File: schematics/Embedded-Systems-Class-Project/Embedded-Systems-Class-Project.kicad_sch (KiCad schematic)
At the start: 16 parts

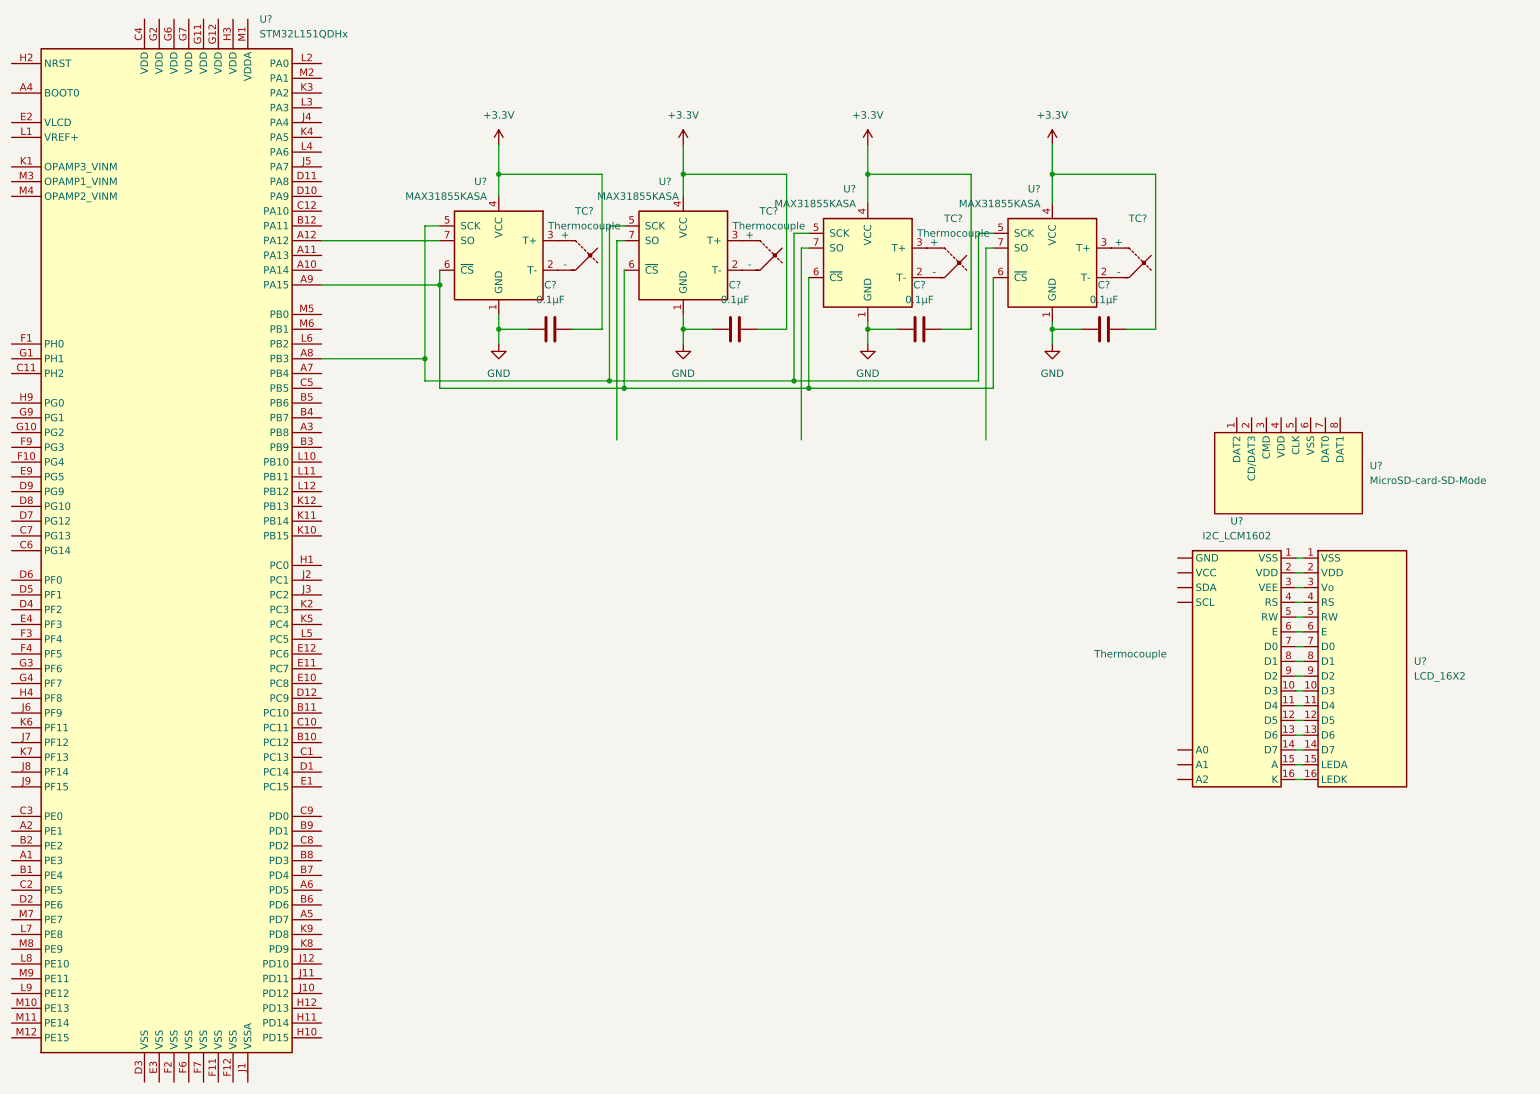
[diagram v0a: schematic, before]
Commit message: updated schematic and library
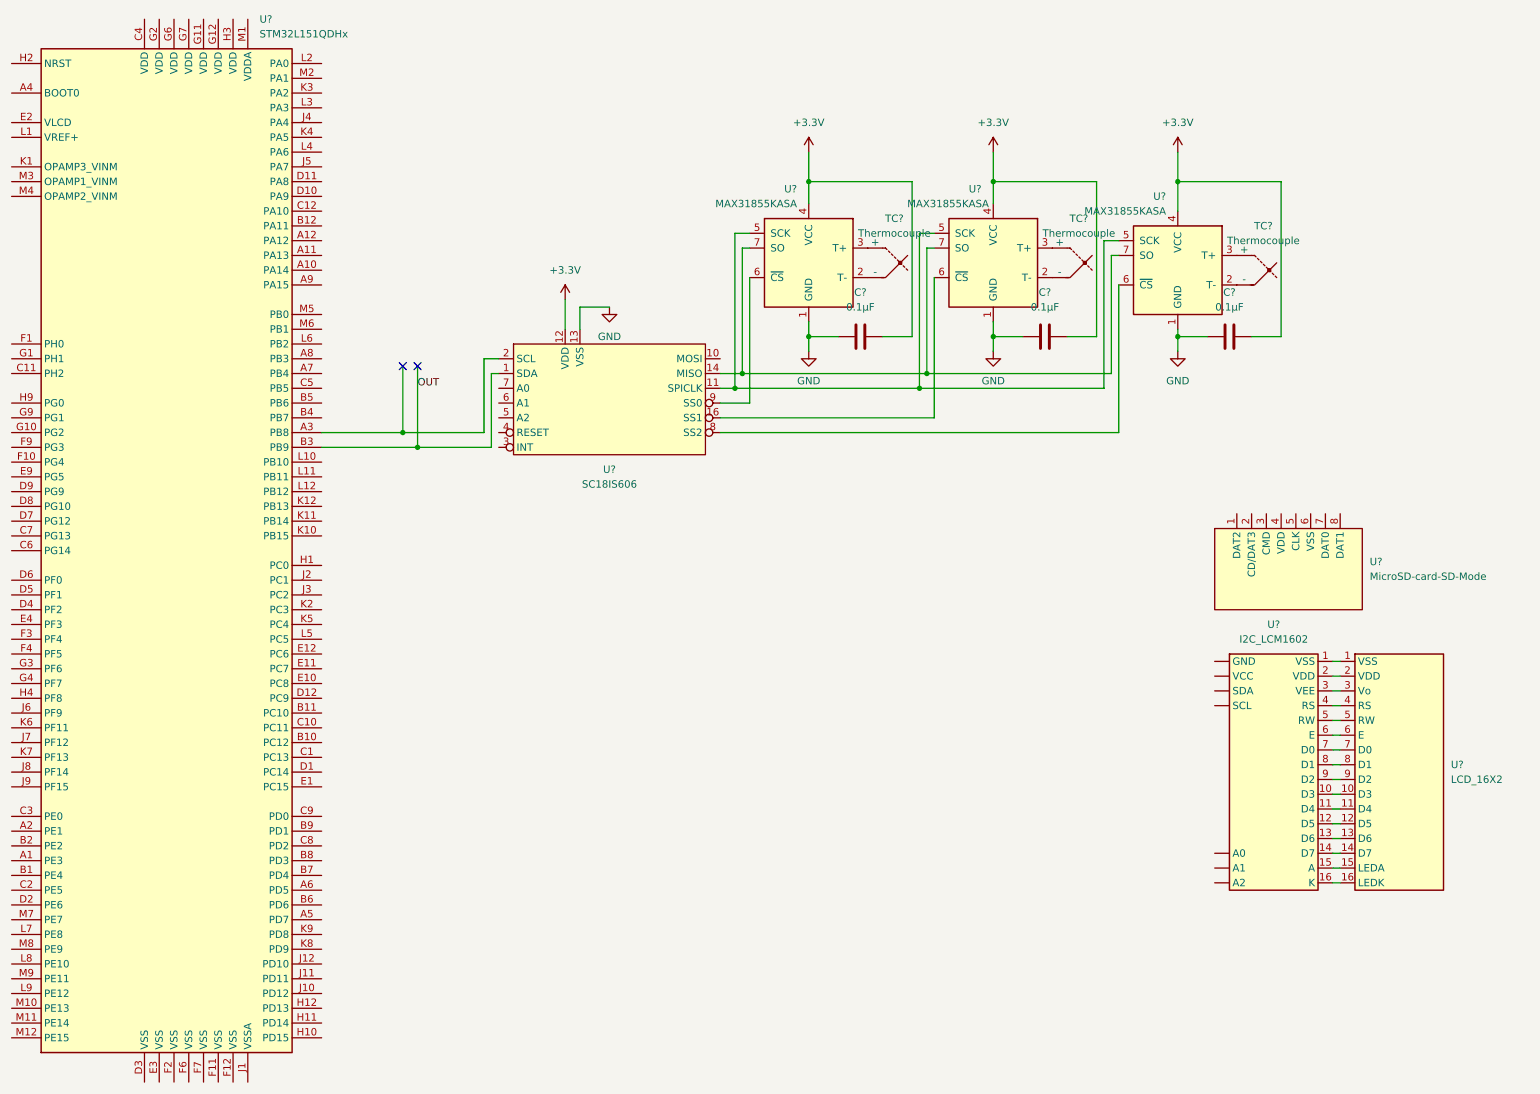
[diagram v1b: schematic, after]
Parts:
- removed C?: 0.1μF, symbol Device:C
- removed TC?: Thermocouple, symbol Device:Thermocouple
- removed U?: MAX31855KASA, Package_SO:SOIC-8_3.9x4.9mm_P1.27mm, symbol Sensor_Temperature:MAX31855KASA
- added U?: SC18IS606, symbol Embedded-Systems-Class-Project:SC18IS606
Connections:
- net +3.3V: now also U?.12 (VDD)
- net GND: now also U?.13 (VSS)
- net at U?.5 (SCK), U?.5 (SCK), U?.5 (SCK): now also U?.11 (SPICLK); no longer U?.A8 (PB3)
- net at U?.7 (SO): now also U?.7 (SO), U?.7 (SO), U?.14 (MISO)
- net at U?.A12 (PA12): no longer U?.7 (SO)
- net at U?.A3 (PB8): now also U?.2 (SCL)
- net OUT: now reaches U?.B3 (PB9)
- net OUT: now also U?.1 (SDA)
- new net: U?.16 (SS1), U?.6 (~{CS})
- new net: U?.6 (~{CS}), U?.8 (SS2)
- new net: U?.6 (~{CS}), U?.9 (SS0)
- now unconnected: U?.A9 (PA15)
- no-connect marks 0 -> 2
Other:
- moved on the sheet: C?, TC?, U?
